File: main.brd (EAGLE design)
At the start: 69.5 x 27.9 mm, 5 parts, among them U1 ATMEGA328P_PDIP

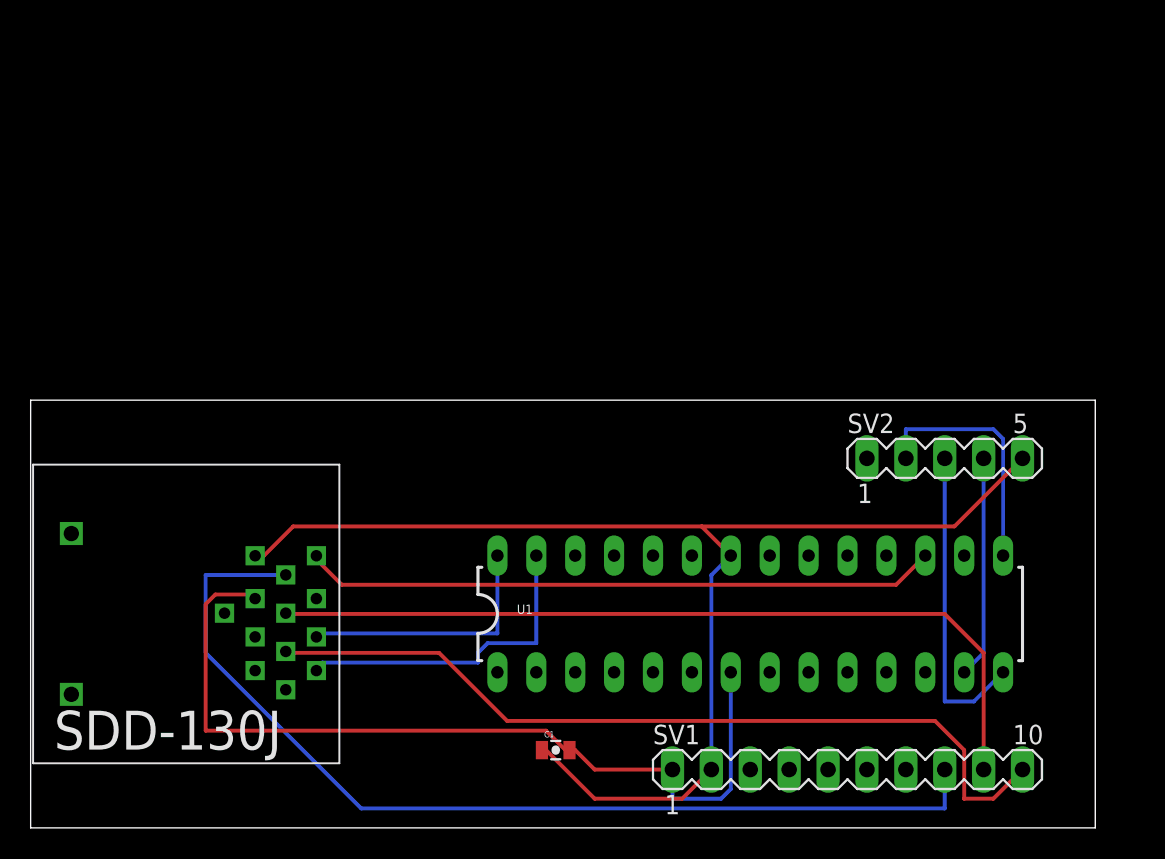
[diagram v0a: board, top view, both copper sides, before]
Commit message: Added files via upload
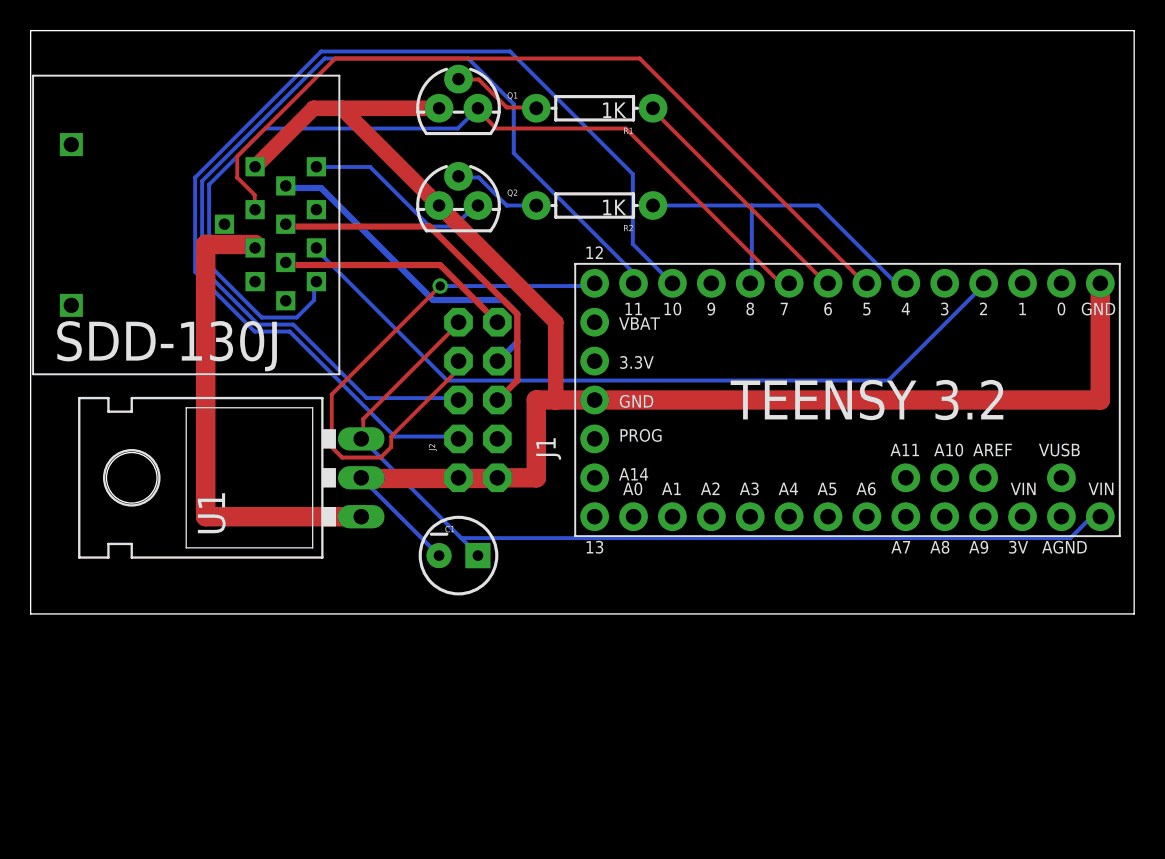
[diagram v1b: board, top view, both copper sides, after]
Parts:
- removed SV1: BT HEADER, con-lstb:MA10-1
- removed SV2: (no value), con-lstb:MA05-1
- added J1: TEENSY-3.1SILK, SparkFun-Boards:TEENSY-3.1
- added J2: (no value), SparkFun-Connectors:2X5_NOSILK
- added Q1, Q2: (no value), SparkFun-DiscreteSemi:TO-92
- added R1, R2: 1K, SparkFun-Resistors:AXIAL-0.3
- C1: value 10UF -> (none); device SparkFun-Capacitors:0805-CAP -> SparkFun-Capacitors:CPOL-RADIAL-10UF-25V
- U1: value ATMEGA328P_PDIP -> (none); device SparkFun-DigitalIC:DIL28-3 -> SparkFun-PowerIC:TO-220-ALT
- moved U1 30.5 mm to (17.8, 50.8), turned to 90 degrees
- moved U$1 25.4 mm to (10.2, 67.3)
- moved C1 14.2 mm to (27.9, 45.7)
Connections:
- removed net LA: SV1.9, U$1.PIN7
- removed net N$10: SV2.3, U1.14
- removed net N$11: SV2.2, U1.15
- removed net N$3: U$1.PIN4, U1.17
- removed net N$5: C1.2, SV1.1, U$1.PIN11, U1.7
- removed net N$9: SV2.4, U1.13
- removed net RA: SV1.8, U$1.PIN8
- removed net SIG: SV1.10, U$1.PIN6
- new net 12VIN: U$1.PIN10, U1.IN
- new net 5VIN: C1.1, J1.VIN, J2.1, U1.OUT
- new net AGND: J2.2, U$1.PIN6
- new net BTC-NX: J1.11, J2.5
- new net BTC-PL: J1.12, J2.3
- new net BTC-PR: J1.10, J2.7
- new net LAUD: J2.4, U$1.PIN8
- new net RAUD: J2.6, U$1.PIN7
- new net REM: J1.5, U$1.PIN11
- new net SCL: J1.2, U$1.PIN2
- new net SDA: J1.7, Q1.3, U$1.PIN1
- new net SDA-O: J1.6, R1.P$1
- new net SRQ: Q2.3, U$1.PIN4
- new net SRQ-D: J1.8, R2.P$1
- net GND: now also C1.2, J1.GND, J1.GND1, J2.10, J2.9, Q1.1, Q2.1, U1.GND; no longer C1.1, SV1.2, SV2.5, U1.22
- net N$1: now also Q1.2, R1.P$2; no longer U$1.PIN1, U1.27
- net N$2: now also Q2.2, R2.P$2; no longer U$1.PIN2, U1.28
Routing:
- net BTC-PR: track 0.00 -> 71.4 mm
- net BTC-NX: track 0.00 -> 65.9 mm
- net RA: track 65.3 -> 0.00 mm
- net 5VIN: track 0.00 -> 63.3 mm
- net SDA: track 0.00 -> 60.0 mm
- net N$5: track 57.1 -> 0.00 mm
- net SIG: track 54.7 -> 0.00 mm
- net LA: track 54.2 -> 0.00 mm
- net REM: track 0.00 -> 53.8 mm
- net SCL: track 0.00 -> 49.9 mm
- net N$3: track 41.4 -> 0.00 mm
- net BTC-PL: track 0.00 -> 35.6 mm, vias 0 -> 1
- net 12VIN: track 0.00 -> 31.4 mm
- net RAUD: track 0.00 -> 23.8 mm
- net SRQ-D: track 0.00 -> 23.7 mm
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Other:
- board size 69.5 x 27.9 mm -> 72.1 x 38.1 mm
- board text added: "Rob Lester V 0.1 BT900"
- board text added: "TEENSY 3.2"
